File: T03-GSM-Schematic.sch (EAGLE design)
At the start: 22 parts, among them IC1 788TV, J1 POWER_JACKPTH_BREAD, J2 AVR, Q2 16M, U1 ATMEGA328P-PU

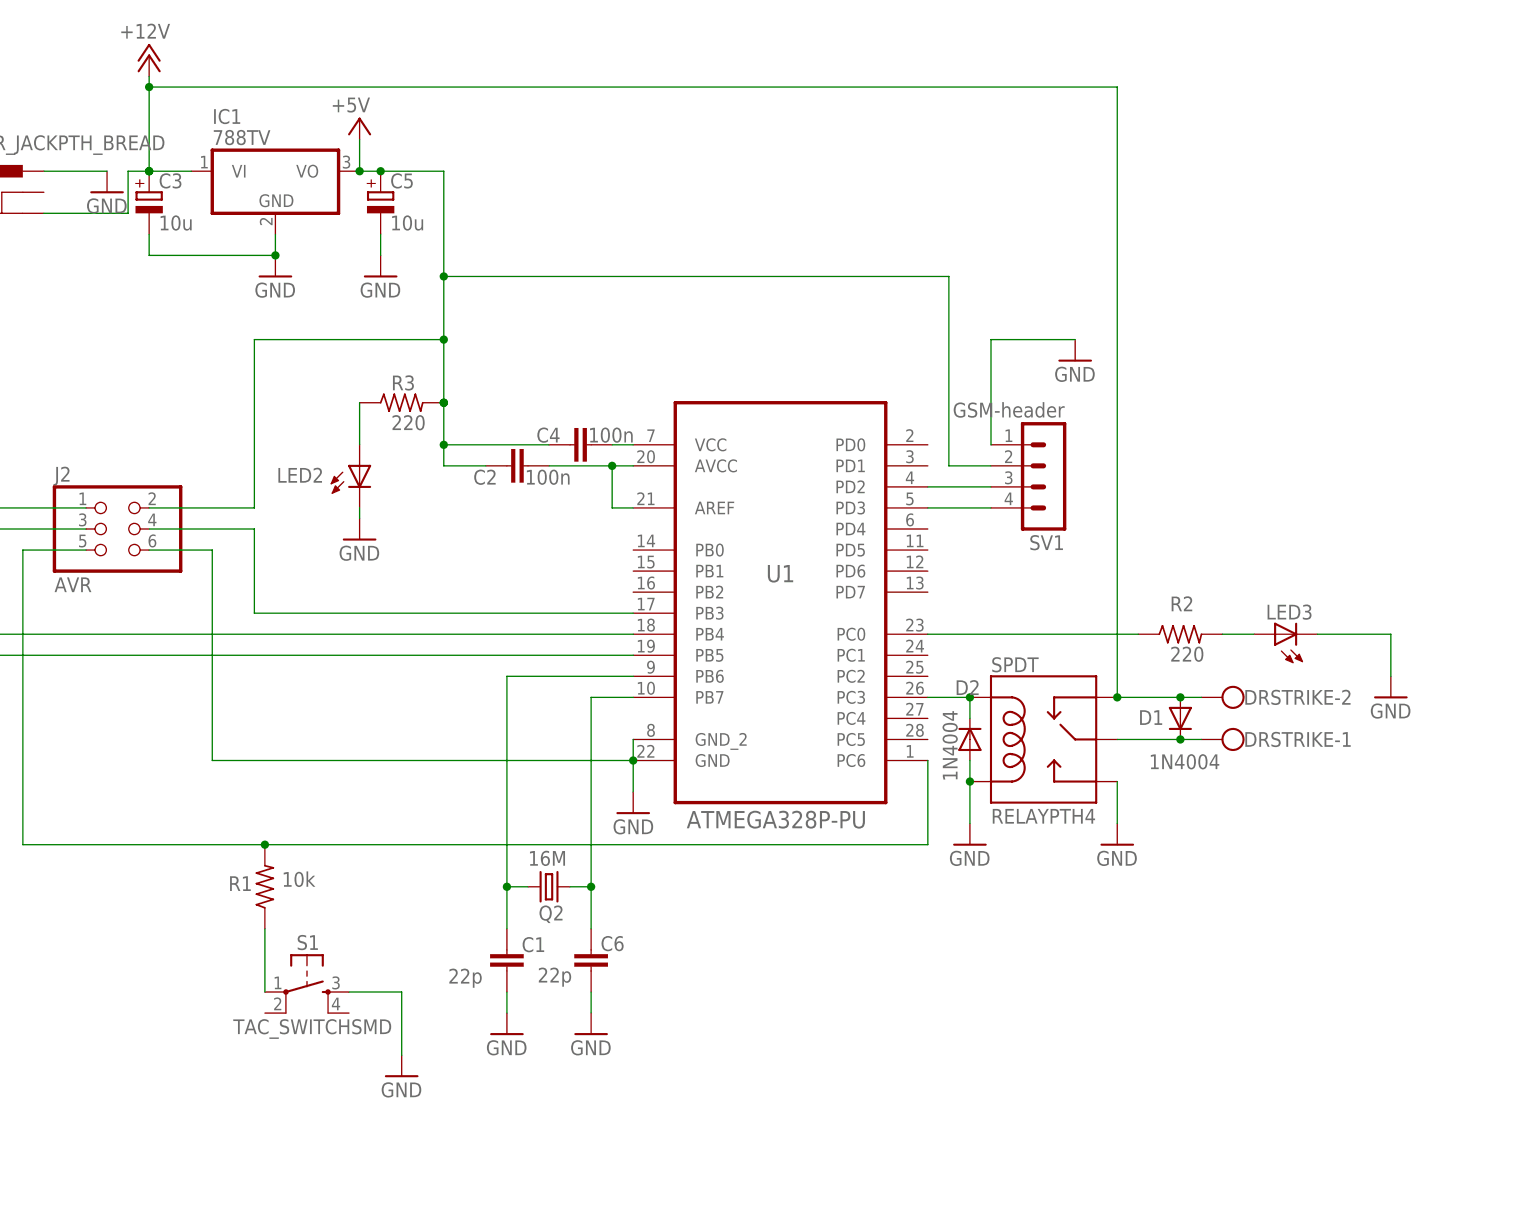
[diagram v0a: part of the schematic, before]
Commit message: Add files via upload
Added test point, fixed ERC error.
More updates to come.
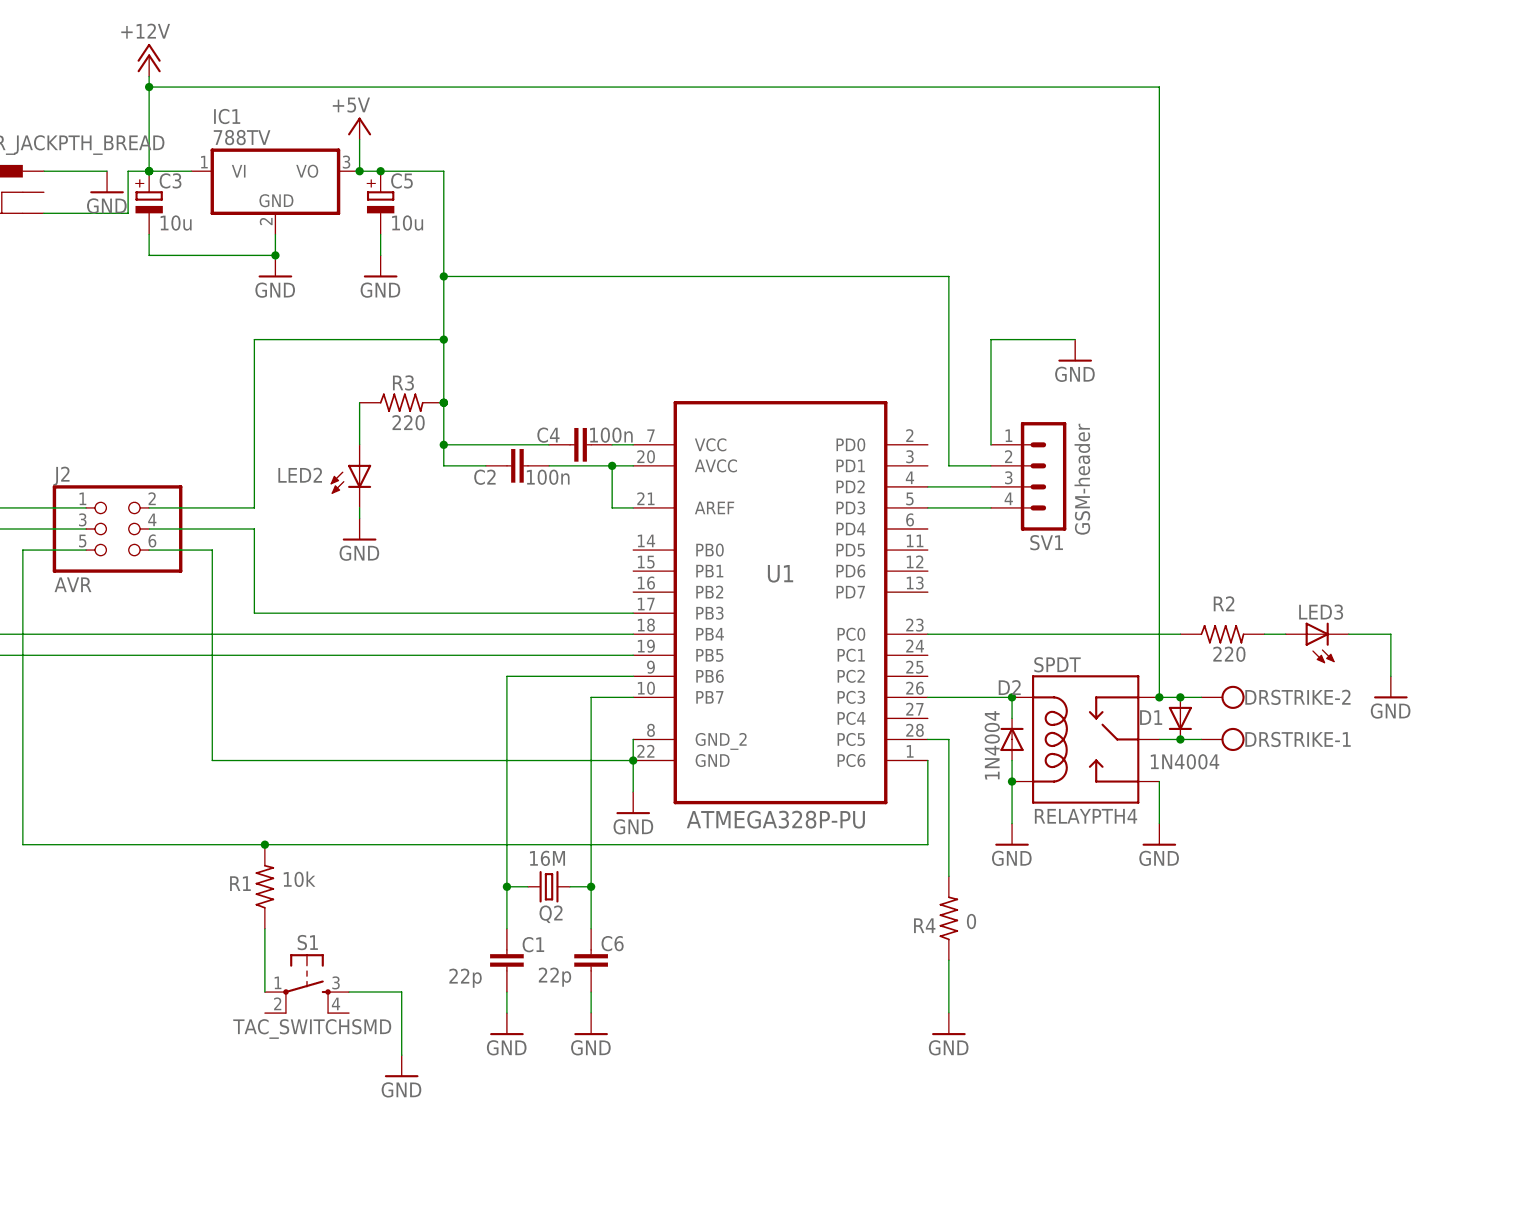
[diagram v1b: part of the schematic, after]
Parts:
- added R4: 0, rcl:R-US_0204/5
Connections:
- new net N$12: R4.2, U1.PC5
- net GND: now also R4.1
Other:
- moved on the sheet: D2, LED3, R2, SPDT
